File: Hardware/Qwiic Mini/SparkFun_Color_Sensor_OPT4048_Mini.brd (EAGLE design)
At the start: 25.4 x 12.7 mm, 51 parts, among them J4 QWIIC_RIGHT_ANGLE, J5 QWIIC_RIGHT_ANGLE, U1 OPT4048

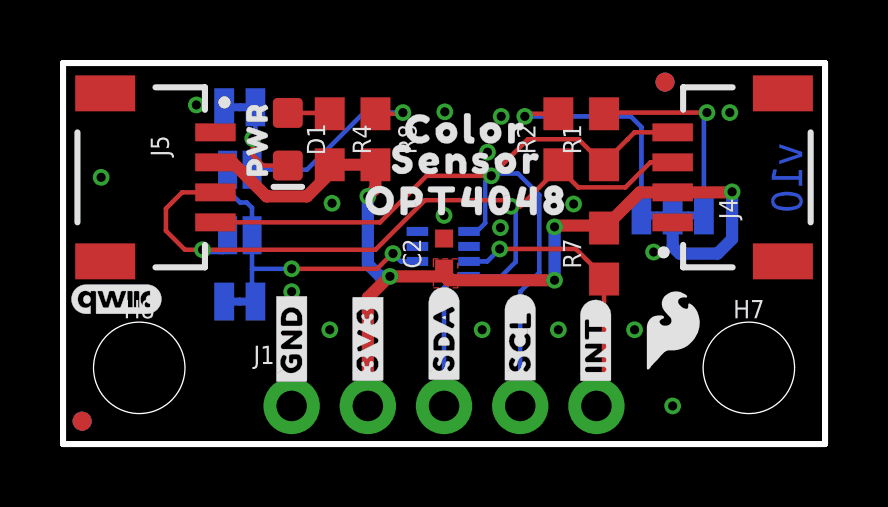
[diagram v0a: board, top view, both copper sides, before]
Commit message: Adds jumper to interrupt pin on both designs
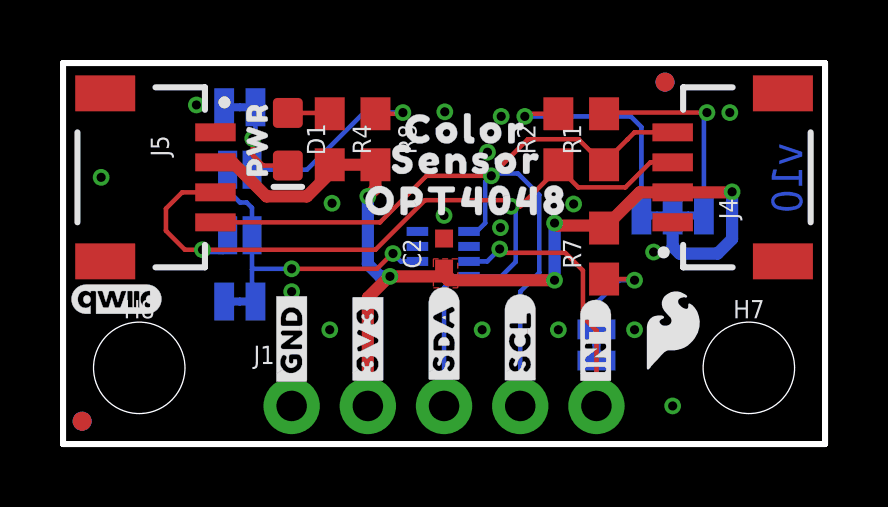
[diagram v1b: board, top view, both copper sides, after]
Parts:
- added INT: JUMPER-SMT_2_NC_TRACE_SILK, SparkFun-Jumpers:SMT-JUMPER_2_NC_TRACE_SILK
- moved U$15 8.07 mm to (23.9, 11.2)
- moved U$7 2.41 mm to (17.8, 5.71)
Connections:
- new net N$5: INT.2, R7.1
- net INT: now also INT.1; no longer R7.1
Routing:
- net N$5: track 0.00 -> 3.49 mm, vias 0 -> 1
- net INT: track 9.46 -> 10.5 mm
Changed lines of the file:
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@@
 <layer number="37" name="tTest" color="7" fill="1" visible="no" active="yes"/>
 <layer number="38" name="bTest" color="7" fill="1" visible="no" active="yes"/>
-<layer number="39" name="tKeepout" color="4" fill="11" visible="no" active="yes"/>
+<layer number="39" name="tKeepout" color="4" fill="11" visible="yes" active="yes"/>
 <layer number="40" name="bKeepout" color="1" fill="11" visible="no" active="yes"/>
 <layer number="41" name="tRestrict" color="4" fill="10" visible="no" active="yes"/>
@@
 <element name="LOGO2" library="SparkFun-Aesthetics" package="QWIIC_3MM" value="QWIIC_LOGO_3MM" x="1.778" y="4.826" smashed="yes"/>
 <element name="LOGO3" library="SparkFun-Aesthetics" package="DUMMY" value="OSHW-LOGONO_SILK" x="-14.478" y="-16.764" smashed="yes"/>
-<element name="U$15" library="SparkFun-Aesthetics" package="OSHW-LOGO-MINI" value="" x="20.32" y="3.937" smashed="yes" rot="MR0"/>
+<element name="U$15" library="SparkFun-Aesthetics" package="OSHW-LOGO-MINI" value="" x="23.876" y="11.176" smashed="yes" rot="MR0"/>
 <element name="R1" library="SparkFun-Resistors" package="0603" value="2.2k" x="18.034" y="10.16" smashed="yes" rot="R90">
 <attribute name="NAME" x="17.272" y="10.16" size="0.6096" layer="25" font="vector" ratio="20" rot="R90" align="bottom-center"/>
@@
 <element name="U$3" library="top_small" package="OPT4048229" value="" x="12.7" y="8.255" smashed="yes" rot="MR0"/>
 <element name="U$8" library="SparkFun-Aesthetics" package="SFE_LOGO_NAME_.1" value="" x="12.7" y="11.049" smashed="yes" rot="MR0"/>
-<element name="U$7" library="bot_small" package="#INT#3" value="" x="17.78" y="3.302" smashed="yes" rot="MR270"/>
+<element name="U$7" library="bot_small" package="#INT#3" value="" x="17.78" y="5.715" smashed="yes" rot="MR270"/>
 <element name="U$9" library="bot_small" package="COLOR14" value="" x="13.4366" y="10.4902" smashed="yes"/>
 <element name="U$11" library="bot_small" package="SENSOR15" value="" x="13.462" y="9.4742" smashed="yes"/>
@@
 <element name="U$6" library="bot_small" package="#0X45#11" value="" x="3.2512" y="9.0932" smashed="yes" rot="MR0"/>
 <element name="U$14" library="bot_small" package="#LED#11" value="" x="3.3782" y="11.2776" smashed="yes" rot="MR0"/>
+<element name="INT" library="SparkFun-Jumpers" package="SMT-JUMPER_2_NC_TRACE_SILK" package3d_urn="urn:adsk.eagle:package:39281/1" value="JUMPER-SMT_2_NC_TRACE_SILK" x="17.78" y="3.302" smashed="yes" rot="MR90">
+<attribute name="NAME" x="18.923" y="3.302" size="0.6096" layer="26" font="vector" ratio="20" rot="MR90" align="bottom-center"/>
+<attribute name="VALUE" x="16.637" y="3.302" size="0.6096" layer="28" font="vector" ratio="20" rot="MR90" align="top-center"/>
+</element>
 </elements>
 <signals>
@@
 <wire x1="19.224" y1="8.39" x2="20.32" y2="8.39" width="0.4064" layer="1"/>
 <via x="16.383" y="5.461" extent="1-16" drill="0.3048"/>
-<wire x1="16.383" y1="5.461" x2="16.383" y2="7.239" width="0.4064" layer="16"/>
-<via x="16.383" y="7.239" extent="1-16" drill="0.3048"/>
-<wire x1="16.383" y1="7.239" x2="16.427" y2="7.283" width="0.4064" layer="1"/>
-<wire x1="16.427" y1="7.283" x2="18.117" y2="7.283" width="0.4064" layer="1"/>
+<wire x1="16.383" y1="5.461" x2="16.383" y2="7.366" width="0.4064" layer="16"/>
+<via x="16.383" y="7.366" extent="1-16" drill="0.3048"/>
+<wire x1="16.383" y1="7.366" x2="16.466" y2="7.283" width="0.4064" layer="1"/>
+<wire x1="16.466" y1="7.283" x2="18.117" y2="7.283" width="0.4064" layer="1"/>
 <wire x1="20.32" y1="8.39" x2="22.2838" y2="8.39" width="0.4064" layer="1"/>
 <wire x1="22.2838" y1="8.39" x2="22.3012" y2="8.4074" width="0.4064" layer="1"/>
@@
 <wire x1="14.0716" y1="8.7376" x2="14.0716" y2="7.366" width="0.1524" layer="16"/>
 <via x="14.2748" y="8.9408" extent="1-16" drill="0.3048"/>
-<wire x1="15.24" y1="1.27" x2="15.24" y2="5.08" width="0.1524" layer="16"/>
+<wire x1="15.24" y1="1.27" x2="15.24" y2="2.54" width="0.1524" layer="16"/>
+<wire x1="15.24" y1="2.54" x2="15.24" y2="5.08" width="0.1524" layer="16"/>
 <wire x1="15.875" y1="5.715" x2="15.875" y2="8.3058" width="0.1524" layer="16"/>
 <wire x1="15.875" y1="8.3058" x2="15.1638" y2="9.017" width="0.1524" layer="16"/>
@@
 <signal name="INT">
 <contactref element="U1" pad="P7"/>
-<contactref element="R7" pad="1"/>
 <contactref element="J1" pad="5"/>
 <wire x1="13.531" y1="6.088" x2="14.1398" y2="6.088" width="0.1524" layer="16"/>
 <wire x1="14.1398" y1="6.088" x2="14.5542" y2="6.5024" width="0.1524" layer="16"/>
 <via x="14.5542" y="6.5024" extent="1-16" drill="0.3048"/>
-<wire x1="17.0942" y1="6.5024" x2="18.034" y2="5.5626" width="0.1524" layer="1"/>
-<wire x1="18.034" y1="5.5626" x2="18.034" y2="5.5" width="0.1524" layer="1"/>
-<wire x1="14.5542" y1="6.5024" x2="17.0942" y2="6.5024" width="0.1524" layer="1"/>
-<wire x1="18.034" y1="5.5" x2="18.034" y2="1.524" width="0.1524" layer="1"/>
-<wire x1="18.034" y1="1.524" x2="17.78" y2="1.27" width="0.1524" layer="1"/>
+<contactref element="INT" pad="1"/>
+<wire x1="17.78" y1="1.27" x2="17.78" y2="2.7813" width="0.1524" layer="16"/>
+<wire x1="16.7386" y1="6.3754" x2="14.6812" y2="6.3754" width="0.1524" layer="1"/>
+<wire x1="14.5542" y1="6.5024" x2="14.6812" y2="6.3754" width="0.1524" layer="1"/>
+<wire x1="17.3308" y1="5.7832" x2="17.3308" y2="4.23083125" width="0.1524" layer="1"/>
+<wire x1="17.78" y1="3.78163125" x2="17.78" y2="1.27" width="0.1524" layer="1"/>
+<wire x1="17.3308" y1="4.23083125" x2="17.78" y2="3.78163125" width="0.1524" layer="1"/>
+<wire x1="16.7386" y1="6.3754" x2="17.3308" y2="5.7832" width="0.1524" layer="1"/>
 </signal>
 <signal name="ADDR">
@@
 <wire x1="8.128" y1="9.144" x2="10.033" y2="11.049" width="0.1524" layer="16"/>
 </signal>
+<signal name="N$5">
+<contactref element="INT" pad="2"/>
+<contactref element="R7" pad="1"/>
+<via x="19.05" y="5.461" extent="1-16" drill="0.3048"/>
+<wire x1="17.78" y1="3.8227" x2="17.78" y2="4.699" width="0.1524" layer="16"/>
+<wire x1="18.542" y1="5.461" x2="19.05" y2="5.461" width="0.1524" layer="16"/>
+<wire x1="17.78" y1="4.699" x2="18.542" y2="5.461" width="0.1524" layer="16"/>
+<wire x1="18.034" y1="5.5" x2="19.011" y2="5.5" width="0.1524" layer="1"/>
+<wire x1="19.011" y1="5.5" x2="19.05" y2="5.461" width="0.1524" layer="1"/>
+</signal>
 </signals>

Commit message: Revert "Adds jumper to interrupt pin on both designs"
This reverts commit a39334068ad88ec2875ce3e39fad74091b9d5839.
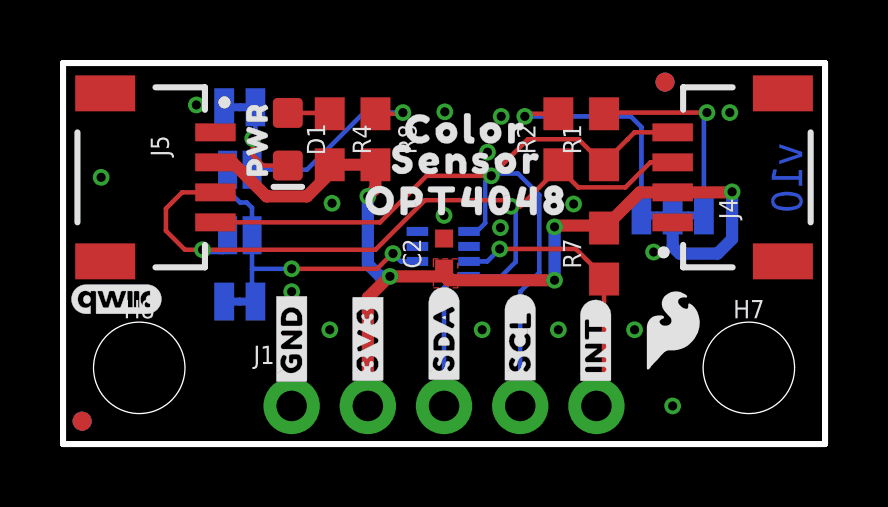
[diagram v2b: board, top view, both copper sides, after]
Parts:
- removed INT: JUMPER-SMT_2_NC_TRACE_SILK, SparkFun-Jumpers:SMT-JUMPER_2_NC_TRACE_SILK
- moved U$15 8.07 mm to (20.3, 3.94)
- moved U$7 2.41 mm to (17.8, 3.30)
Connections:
- removed net N$5: INT.2, R7.1
- net INT: now also R7.1; no longer INT.1
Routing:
- net N$5: track 3.49 -> 0.00 mm, vias 1 -> 0
- net INT: track 10.5 -> 9.46 mm
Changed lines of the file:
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@@
 <layer number="37" name="tTest" color="7" fill="1" visible="no" active="yes"/>
 <layer number="38" name="bTest" color="7" fill="1" visible="no" active="yes"/>
-<layer number="39" name="tKeepout" color="4" fill="11" visible="yes" active="yes"/>
+<layer number="39" name="tKeepout" color="4" fill="11" visible="no" active="yes"/>
 <layer number="40" name="bKeepout" color="1" fill="11" visible="no" active="yes"/>
 <layer number="41" name="tRestrict" color="4" fill="10" visible="no" active="yes"/>
@@
 <element name="LOGO2" library="SparkFun-Aesthetics" package="QWIIC_3MM" value="QWIIC_LOGO_3MM" x="1.778" y="4.826" smashed="yes"/>
 <element name="LOGO3" library="SparkFun-Aesthetics" package="DUMMY" value="OSHW-LOGONO_SILK" x="-14.478" y="-16.764" smashed="yes"/>
-<element name="U$15" library="SparkFun-Aesthetics" package="OSHW-LOGO-MINI" value="" x="23.876" y="11.176" smashed="yes" rot="MR0"/>
+<element name="U$15" library="SparkFun-Aesthetics" package="OSHW-LOGO-MINI" value="" x="20.32" y="3.937" smashed="yes" rot="MR0"/>
 <element name="R1" library="SparkFun-Resistors" package="0603" value="2.2k" x="18.034" y="10.16" smashed="yes" rot="R90">
 <attribute name="NAME" x="17.272" y="10.16" size="0.6096" layer="25" font="vector" ratio="20" rot="R90" align="bottom-center"/>
@@
 <element name="U$3" library="top_small" package="OPT4048229" value="" x="12.7" y="8.255" smashed="yes" rot="MR0"/>
 <element name="U$8" library="SparkFun-Aesthetics" package="SFE_LOGO_NAME_.1" value="" x="12.7" y="11.049" smashed="yes" rot="MR0"/>
-<element name="U$7" library="bot_small" package="#INT#3" value="" x="17.78" y="5.715" smashed="yes" rot="MR270"/>
+<element name="U$7" library="bot_small" package="#INT#3" value="" x="17.78" y="3.302" smashed="yes" rot="MR270"/>
 <element name="U$9" library="bot_small" package="COLOR14" value="" x="13.4366" y="10.4902" smashed="yes"/>
 <element name="U$11" library="bot_small" package="SENSOR15" value="" x="13.462" y="9.4742" smashed="yes"/>
@@
 <element name="U$6" library="bot_small" package="#0X45#11" value="" x="3.2512" y="9.0932" smashed="yes" rot="MR0"/>
 <element name="U$14" library="bot_small" package="#LED#11" value="" x="3.3782" y="11.2776" smashed="yes" rot="MR0"/>
-<element name="INT" library="SparkFun-Jumpers" package="SMT-JUMPER_2_NC_TRACE_SILK" package3d_urn="urn:adsk.eagle:package:39281/1" value="JUMPER-SMT_2_NC_TRACE_SILK" x="17.78" y="3.302" smashed="yes" rot="MR90">
-<attribute name="NAME" x="18.923" y="3.302" size="0.6096" layer="26" font="vector" ratio="20" rot="MR90" align="bottom-center"/>
-<attribute name="VALUE" x="16.637" y="3.302" size="0.6096" layer="28" font="vector" ratio="20" rot="MR90" align="top-center"/>
-</element>
 </elements>
 <signals>
@@
 <wire x1="19.224" y1="8.39" x2="20.32" y2="8.39" width="0.4064" layer="1"/>
 <via x="16.383" y="5.461" extent="1-16" drill="0.3048"/>
-<wire x1="16.383" y1="5.461" x2="16.383" y2="7.366" width="0.4064" layer="16"/>
-<via x="16.383" y="7.366" extent="1-16" drill="0.3048"/>
-<wire x1="16.383" y1="7.366" x2="16.466" y2="7.283" width="0.4064" layer="1"/>
-<wire x1="16.466" y1="7.283" x2="18.117" y2="7.283" width="0.4064" layer="1"/>
+<wire x1="16.383" y1="5.461" x2="16.383" y2="7.239" width="0.4064" layer="16"/>
+<via x="16.383" y="7.239" extent="1-16" drill="0.3048"/>
+<wire x1="16.383" y1="7.239" x2="16.427" y2="7.283" width="0.4064" layer="1"/>
+<wire x1="16.427" y1="7.283" x2="18.117" y2="7.283" width="0.4064" layer="1"/>
 <wire x1="20.32" y1="8.39" x2="22.2838" y2="8.39" width="0.4064" layer="1"/>
 <wire x1="22.2838" y1="8.39" x2="22.3012" y2="8.4074" width="0.4064" layer="1"/>
@@
 <wire x1="14.0716" y1="8.7376" x2="14.0716" y2="7.366" width="0.1524" layer="16"/>
 <via x="14.2748" y="8.9408" extent="1-16" drill="0.3048"/>
-<wire x1="15.24" y1="1.27" x2="15.24" y2="2.54" width="0.1524" layer="16"/>
-<wire x1="15.24" y1="2.54" x2="15.24" y2="5.08" width="0.1524" layer="16"/>
+<wire x1="15.24" y1="1.27" x2="15.24" y2="5.08" width="0.1524" layer="16"/>
 <wire x1="15.875" y1="5.715" x2="15.875" y2="8.3058" width="0.1524" layer="16"/>
 <wire x1="15.875" y1="8.3058" x2="15.1638" y2="9.017" width="0.1524" layer="16"/>
@@
 <signal name="INT">
 <contactref element="U1" pad="P7"/>
+<contactref element="R7" pad="1"/>
 <contactref element="J1" pad="5"/>
 <wire x1="13.531" y1="6.088" x2="14.1398" y2="6.088" width="0.1524" layer="16"/>
 <wire x1="14.1398" y1="6.088" x2="14.5542" y2="6.5024" width="0.1524" layer="16"/>
 <via x="14.5542" y="6.5024" extent="1-16" drill="0.3048"/>
-<contactref element="INT" pad="1"/>
-<wire x1="17.78" y1="1.27" x2="17.78" y2="2.7813" width="0.1524" layer="16"/>
-<wire x1="16.7386" y1="6.3754" x2="14.6812" y2="6.3754" width="0.1524" layer="1"/>
-<wire x1="14.5542" y1="6.5024" x2="14.6812" y2="6.3754" width="0.1524" layer="1"/>
-<wire x1="17.3308" y1="5.7832" x2="17.3308" y2="4.23083125" width="0.1524" layer="1"/>
-<wire x1="17.78" y1="3.78163125" x2="17.78" y2="1.27" width="0.1524" layer="1"/>
-<wire x1="17.3308" y1="4.23083125" x2="17.78" y2="3.78163125" width="0.1524" layer="1"/>
-<wire x1="16.7386" y1="6.3754" x2="17.3308" y2="5.7832" width="0.1524" layer="1"/>
+<wire x1="17.0942" y1="6.5024" x2="18.034" y2="5.5626" width="0.1524" layer="1"/>
+<wire x1="18.034" y1="5.5626" x2="18.034" y2="5.5" width="0.1524" layer="1"/>
+<wire x1="14.5542" y1="6.5024" x2="17.0942" y2="6.5024" width="0.1524" layer="1"/>
+<wire x1="18.034" y1="5.5" x2="18.034" y2="1.524" width="0.1524" layer="1"/>
+<wire x1="18.034" y1="1.524" x2="17.78" y2="1.27" width="0.1524" layer="1"/>
 </signal>
 <signal name="ADDR">
@@
 <wire x1="8.128" y1="9.144" x2="10.033" y2="11.049" width="0.1524" layer="16"/>
 </signal>
-<signal name="N$5">
-<contactref element="INT" pad="2"/>
-<contactref element="R7" pad="1"/>
-<via x="19.05" y="5.461" extent="1-16" drill="0.3048"/>
-<wire x1="17.78" y1="3.8227" x2="17.78" y2="4.699" width="0.1524" layer="16"/>
-<wire x1="18.542" y1="5.461" x2="19.05" y2="5.461" width="0.1524" layer="16"/>
-<wire x1="17.78" y1="4.699" x2="18.542" y2="5.461" width="0.1524" layer="16"/>
-<wire x1="18.034" y1="5.5" x2="19.011" y2="5.5" width="0.1524" layer="1"/>
-<wire x1="19.011" y1="5.5" x2="19.05" y2="5.461" width="0.1524" layer="1"/>
-</signal>
 </signals>
